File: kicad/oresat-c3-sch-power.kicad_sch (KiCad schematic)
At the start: 58 parts, among them U31 LP2985AIM5-3.3, U34 TPS259621DDA, U35 TPS259620DDA, U36 LTC3624-5, U6 LTC3624-5

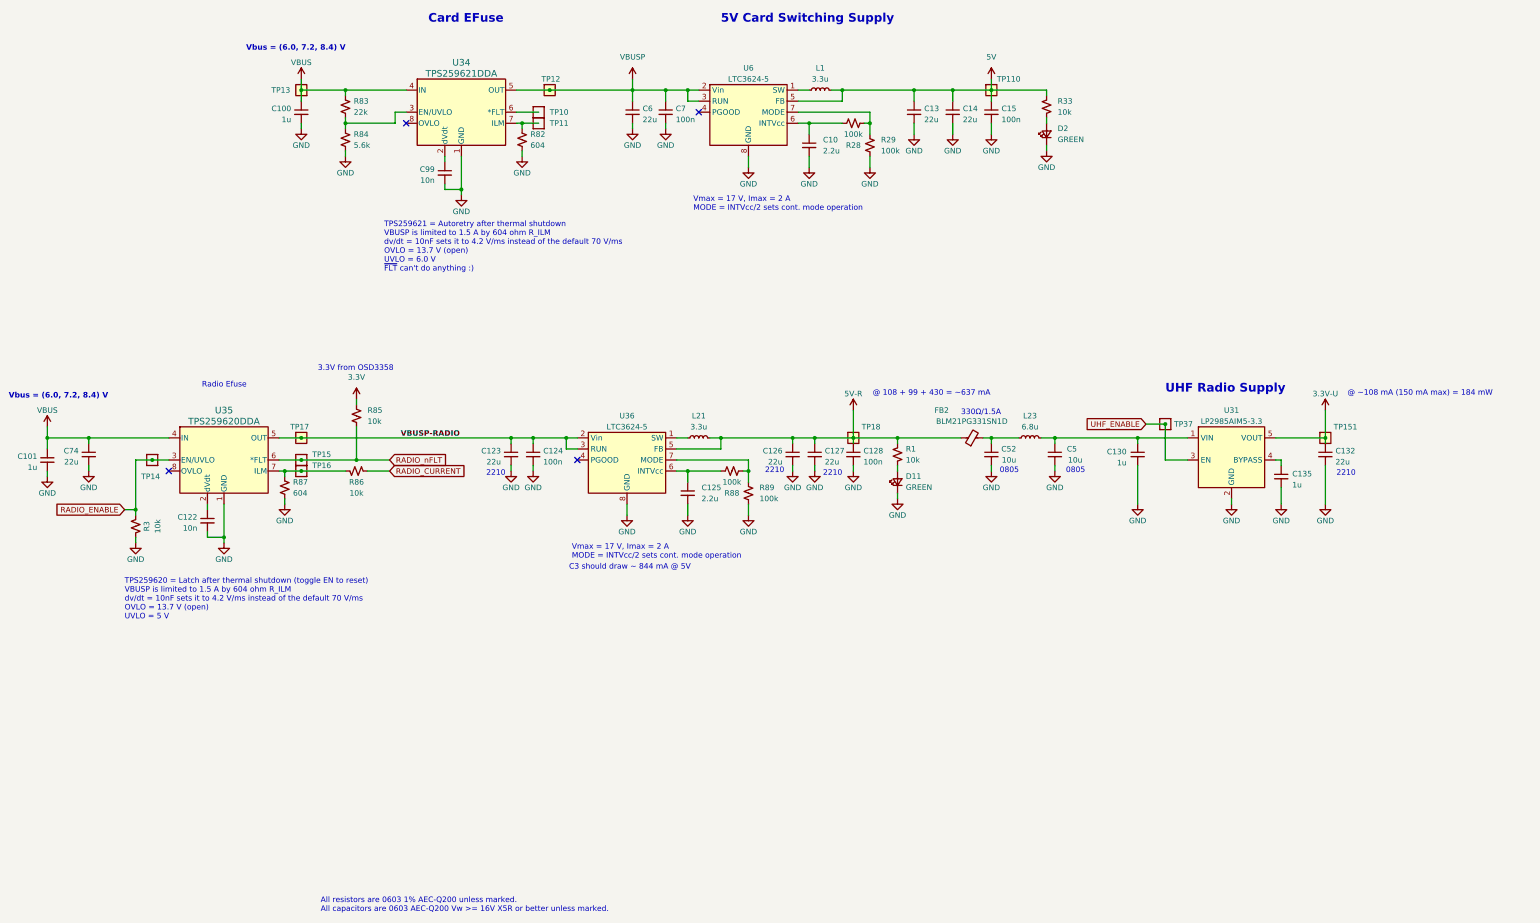
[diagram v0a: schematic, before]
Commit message: Removed power switching circuitry
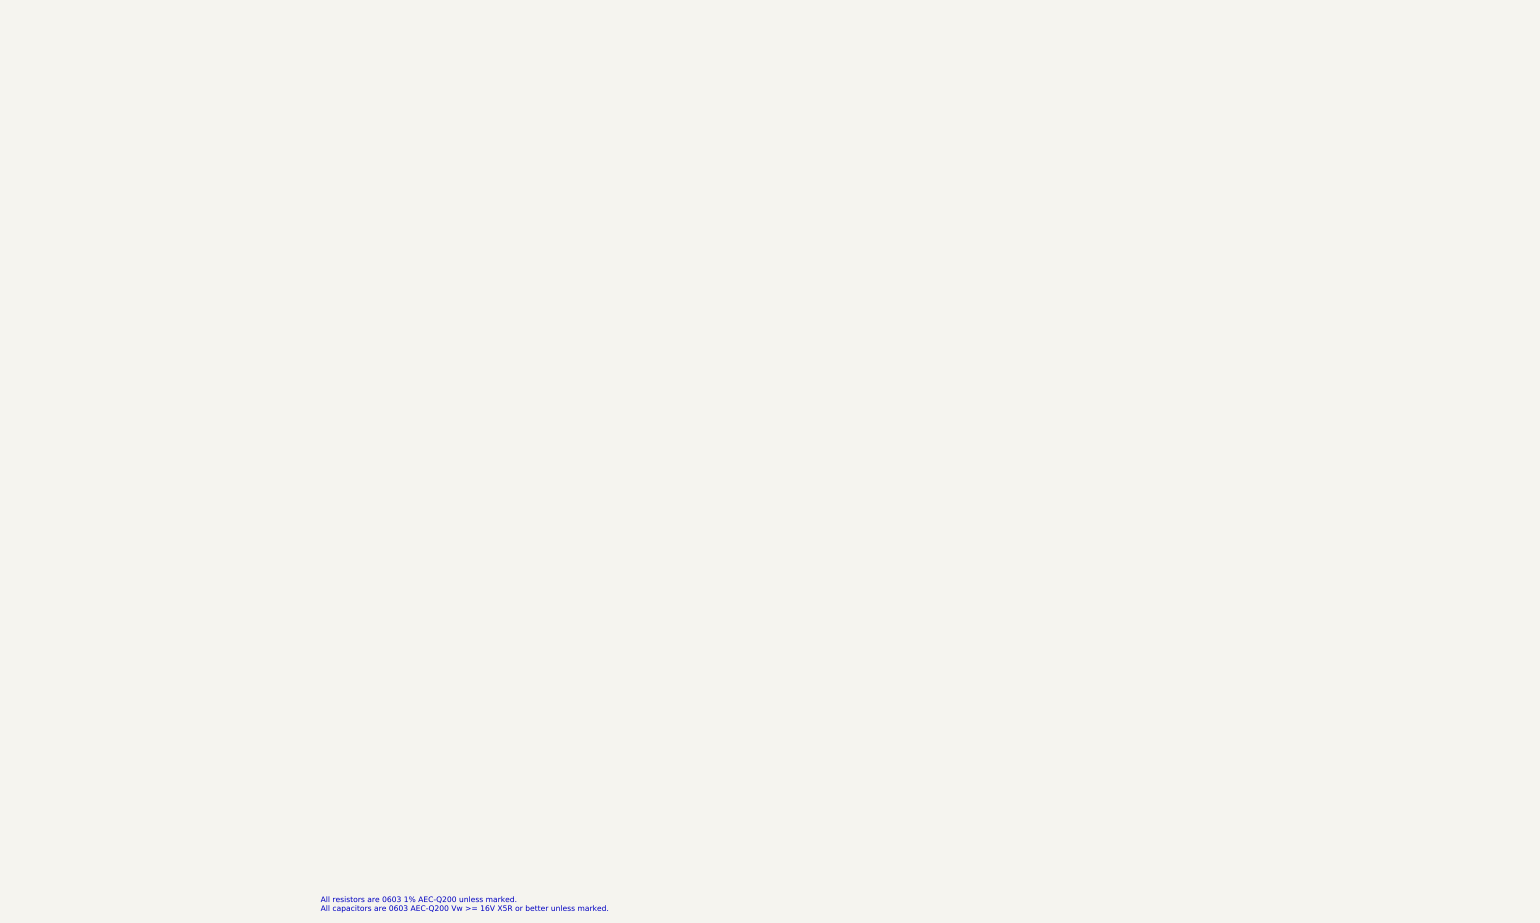
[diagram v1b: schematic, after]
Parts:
- removed C10, C125: 2.2u, Capacitor_SMD:C_0603_1608Metric, symbol Device:C_Small
- removed C100, C101, C130, C135: 1u, Capacitor_SMD:C_0603_1608Metric, symbol Device:C_Small
- removed C122, C99: 10n, Capacitor_SMD:C_0603_1608Metric, symbol Device:C_Small
- removed C123, C126, C127, C13, C132, C14, C6, C74: 22u, Capacitor_SMD:C_1210_3225Metric, symbol Device:C_Small
- removed C124, C128, C15, C7: 100n, Capacitor_SMD:C_0603_1608Metric, symbol Device:C_Small
- removed C5, C52: 10u, Capacitor_SMD:C_0805_2012Metric, symbol Device:C_Small
- removed D11, D2: GREEN, LED_SMD:LED_0603_1608Metric, symbol Device:LED_Small
- removed FB2: BLM21PG331SN1D, Resistor_SMD:R_0805_2012Metric, symbol Device:FerriteBead_Small
- removed L1, L21: 3.3u, oresat-passives:L_ECS-MPI4040, symbol Device:L_Small
- removed L23: 6.8u, oresat-passives:L_ECS-MPI4040, symbol Device:L_Small
- removed R1, R3, R33, R85, R86: 10k, Resistor_SMD:R_0603_1608Metric, symbol Device:R_Small_US
- removed R28, R29, R88, R89: 100k, Resistor_SMD:R_0603_1608Metric, symbol Device:R_Small_US
- removed R82, R87: 604, Resistor_SMD:R_0603_1608Metric, symbol Device:R_Small_US
- removed R83: 22k, Resistor_SMD:R_0603_1608Metric, symbol Device:R_Small_US
- removed R84: 5.6k, Resistor_SMD:R_0603_1608Metric, symbol Device:R_Small_US
- removed TP10, TP11, TP14, TP15, TP16, TP37: Test-Point, oresat-misc:TestPoint_Pad_D1.0mm, symbol oresat-misc:Test-Point-1mm-round
- removed TP110, TP12, TP13, TP151, TP17, TP18: Test-Point, oresat-misc:TestPoint-0.75mm-th, symbol oresat-misc:Test-Point-0.75mm-th
- removed U31: LP2985AIM5-3.3, Package_TO_SOT_SMD:SOT-23-5, symbol oresat-ics:LP2985-N
- removed U34: TPS259621DDA, Package_SO:Texas_R-PDSO-G8_EP2.95x4.9mm_Mask2.4x3.1mm_ThermalVias, symbol oresat-ics:TPS259621DDA
- removed U35: TPS259620DDA, Package_SO:Texas_R-PDSO-G8_EP2.95x4.9mm_Mask2.4x3.1mm_ThermalVias, symbol oresat-ics:TPS259621DDA
- removed U36, U6: LTC3624-5, oresat-ics:DFN-8-1EP_3x3mm_P0.5mm_EP1.65x2.38mm_ThermalVias0.3mm, symbol oresat-ics:LTC3624
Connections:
- no-connect marks 4 -> 0
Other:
- note removed: "0805"
- note removed: "2210"
- note removed: "3.3V from OSD3358"
- note removed: "330Ω/1.5A"
- note removed: "5V Card Switching Supply"
- note removed: "@ 108 + 99 + 430 = ~637 mA"
- note removed: "@ ~108 mA (150 mA max) = 184 mW"
- note removed: "C3 should draw ~ 844 mA @ 5V"
- note removed: "Card EFuse"
- note removed: "Radio Efuse"
- note removed: "TPS259620 = Latch after thermal shutdown (toggle EN to reset) VBUSP is limited to 1.5 A by 604 ohm R_ILM dv/dt = 10nF sets it to 4.2 V/ms instead of the default 70 V/ms OVLO = 13.7 V (open) UVLO = 5 V"
- note removed: "TPS259621 = Autoretry after thermal shutdown VBUSP is limited to 1.5 A by 604 ohm R_ILM dv/dt = 10nF sets it to 4.2 V/ms instead of the default 70 V/ms OVLO = 13.7 V (open) UVLO = 6.0 V ~{FLT} can't do anything :)"
- note removed: "UHF Radio Supply"
- note removed: "Vbus = (6.0, 7.2, 8.4) V"
- note removed: "Vmax = 17 V, Imax = 2 A MODE = INTVcc/2 sets cont. mode operation"
